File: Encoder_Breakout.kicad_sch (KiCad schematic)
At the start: 4 parts, among them J1 Conn_01x03, J2 Conn_02x07_Odd_Even, J3 Conn_01x02, J4 Conn_01x02

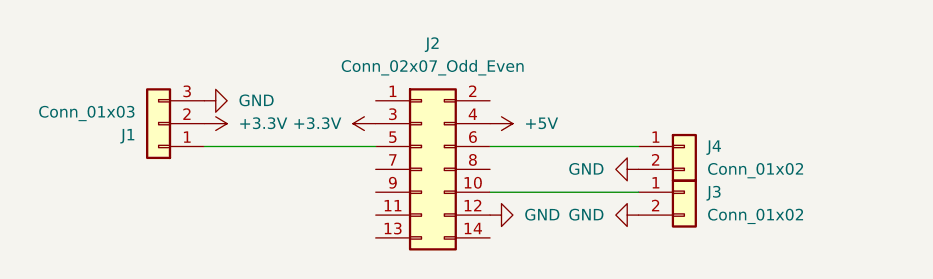
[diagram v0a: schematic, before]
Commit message: PCB changes and add kibot
Signed-off-by: Colin <cfinn68916@gmail.com>
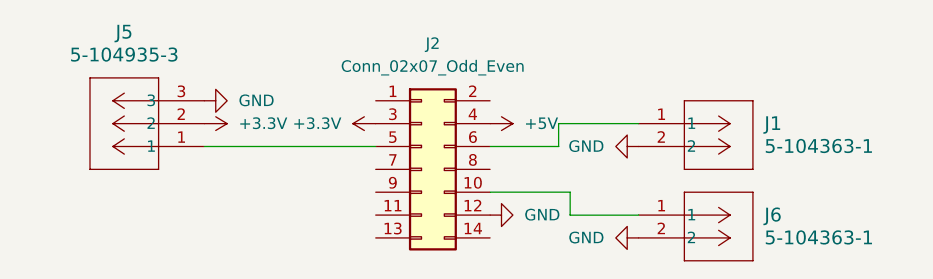
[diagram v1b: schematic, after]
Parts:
- removed J1: Conn_01x03, Connector_PinHeader_2.54mm:PinHeader_1x03_P2.54mm_Horizontal, symbol Connector_Generic:Conn_01x03
- removed J3, J4: Conn_01x02, Connector_PinSocket_2.54mm:PinSocket_1x02_P2.54mm_Vertical, symbol Connector_Generic:Conn_01x02
- added J1, J6: 5-104363-1, CONN_5-104363-1_TYCO, symbol 2023-10-03_23-14-34:5-104363-1
- added J5: 5-104935-3, footprints:CONN_5-104935-3_TYCO, symbol 2023-10-03_22-41-26:5-104935-3
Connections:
- net +3.3V: now also J5.2
- net GND: now also J1.2, J5.3, J6.2
- net at J2.10 (Pin_10): now also J6.1
- net at J2.6 (Pin_6): now also J1.1
- net at J2.5 (Pin_5): now also J5.1
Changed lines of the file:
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@@
 (kicad_sch (version 20230121) (generator eeschema)
   (paper "A4")
-  (wire (pts (xy 146.05 80.01) (xy 162.56 80.01))
+  (wire (pts (xy 154.94 87.63) (xy 162.56 87.63))
+    (stroke (width 0) (type default))
+  )
+  (wire (pts (xy 146.05 80.01) (xy 153.67 80.01))
+    (stroke (width 0) (type default))
+  )
+  (wire (pts (xy 146.05 85.09) (xy 154.94 85.09))
+    (stroke (width 0) (type default))
+  )
+  (wire (pts (xy 154.94 85.09) (xy 154.94 87.63))
+    (stroke (width 0) (type default))
+  )
+  (wire (pts (xy 153.67 80.01) (xy 153.67 77.47))
     (stroke (width 0) (type default))
   )
@@
     (stroke (width 0) (type default))
   )
-  (wire (pts (xy 146.05 85.09) (xy 162.56 85.09))
-    (stroke (width 0) (type default))
-  )
-  (symbol (lib_id "power:GND") (at 162.56 82.55 270) (unit 1)
-    (in_bom yes) (on_board yes) (dnp no) (fields_autoplaced)
-    (property "Reference" "#PWR07" (at 156.21 82.55 0)
-      (effects (font (size 1.27 1.27)) hide)
-    )
-    (property "Value" "GND" (at 158.75 82.55 90)
-      (effects (font (size 1.27 1.27)) (justify right))
-    )
-    (property "Footprint" "" (at 162.56 82.55 0)
-      (effects (font (size 1.27 1.27)) hide)
-    )
-    (property "Datasheet" "" (at 162.56 82.55 0)
+  (wire (pts (xy 153.67 77.47) (xy 162.56 77.47))
+    (stroke (width 0) (type default))
+  )
+  (symbol (lib_id "power:GND") (at 162.56 80.01 270) (unit 1)
+    (in_bom yes) (on_board yes) (dnp no) (fields_autoplaced)
+    (property "Reference" "#PWR07" (at 156.21 80.01 0)
+      (effects (font (size 1.27 1.27)) hide)
+    )
+    (property "Value" "GND" (at 158.75 80.01 90)
+      (effects (font (size 1.27 1.27)) (justify right))
+    )
+    (property "Footprint" "" (at 162.56 80.01 0)
+      (effects (font (size 1.27 1.27)) hide)
+    )
+    (property "Datasheet" "" (at 162.56 80.01 0)
       (effects (font (size 1.27 1.27)) hide)
     )
@@
     )
   )
-  (symbol (lib_id "Connector_Generic:Conn_01x02") (at 167.64 85.09 0) (unit 1)
-    (in_bom yes) (on_board yes) (dnp no) (fields_autoplaced)
-    (property "Reference" "J3" (at 170.18 85.09 0)
-      (effects (font (size 1.27 1.27)) (justify left))
-    )
-    (property "Value" "Conn_01x02" (at 170.18 87.63 0)
-      (effects (font (size 1.27 1.27)) (justify left))
-    )
-    (property "Footprint" "Connector_PinSocket_2.54mm:PinSocket_1x02_P2.54mm_Vertical" (at 167.64 85.09 0)
-      (effects (font (size 1.27 1.27)) hide)
-    )
-    (property "Datasheet" "~" (at 167.64 85.09 0)
-      (effects (font (size 1.27 1.27)) hide)
-    )
-    (pin "1")
-    (pin "2")
-    (instances
-      (project "Encoder_Breakout"
-        (path "/896045ed-d89c-42ad-9d47-a66b46c2187b"
-          (reference "J3") (unit 1)
+  (symbol (lib_id "2023-10-03_23-14-34:5-104363-1") (at 162.56 77.47 0) (unit 1)
+    (in_bom yes) (on_board yes) (dnp no) (fields_autoplaced)
+    (property "Reference" "J1" (at 176.53 77.47 0)
+      (effects (font (size 1.524 1.524)) (justify left))
+    )
+    (property "Value" "5-104363-1" (at 176.53 80.01 0)
+      (effects (font (size 1.524 1.524)) (justify left))
+    )
+    (property "Footprint" "CONN_5-104363-1_TYCO" (at 162.56 77.47 0)
+      (effects (font (size 1.27 1.27) italic) hide)
+    )
+    (property "Datasheet" "5-104363-1" (at 162.56 77.47 0)
+      (effects (font (size 1.27 1.27) italic) hide)
+    )
+    (pin "1")
+    (pin "2")
+    (instances
+      (project "Encoder_Breakout"
+        (path "/896045ed-d89c-42ad-9d47-a66b46c2187b"
+          (reference "J1") (unit 1)
         )
       )
@@
         (path "/896045ed-d89c-42ad-9d47-a66b46c2187b"
           (reference "#PWR05") (unit 1)
-        )
-      )
-    )
-  )
-  (symbol (lib_id "Connector_Generic:Conn_01x02") (at 167.64 80.01 0) (unit 1)
-    (in_bom yes) (on_board yes) (dnp no) (fields_autoplaced)
-    (property "Reference" "J4" (at 170.18 80.01 0)
-      (effects (font (size 1.27 1.27)) (justify left))
-    )
-    (property "Value" "Conn_01x02" (at 170.18 82.55 0)
-      (effects (font (size 1.27 1.27)) (justify left))
-    )
-    (property "Footprint" "Connector_PinSocket_2.54mm:PinSocket_1x02_P2.54mm_Vertical" (at 167.64 80.01 0)
-      (effects (font (size 1.27 1.27)) hide)
-    )
-    (property "Datasheet" "~" (at 167.64 80.01 0)
-      (effects (font (size 1.27 1.27)) hide)
-    )
-    (pin "1")
-    (pin "2")
-    (instances
-      (project "Encoder_Breakout"
-        (path "/896045ed-d89c-42ad-9d47-a66b46c2187b"
-          (reference "J4") (unit 1)
         )
       )
@@
         (path "/896045ed-d89c-42ad-9d47-a66b46c2187b"
           (reference "#PWR04") (unit 1)
-        )
-      )
-    )
-  )
-  (symbol (lib_id "Connector_Generic:Conn_01x03") (at 109.22 77.47 180) (unit 1)
-    (in_bom yes) (on_board yes) (dnp no) (fields_autoplaced)
-    (property "Reference" "J1" (at 106.68 78.74 0)
-      (effects (font (size 1.27 1.27)) (justify left))
-    )
-    (property "Value" "Conn_01x03" (at 106.68 76.2 0)
-      (effects (font (size 1.27 1.27)) (justify left))
-    )
-    (property "Footprint" "Connector_PinHeader_2.54mm:PinHeader_1x03_P2.54mm_Horizontal" (at 109.22 77.47 0)
-      (effects (font (size 1.27 1.27)) hide)
-    )
-    (property "Datasheet" "~" (at 109.22 77.47 0)
-      (effects (font (size 1.27 1.27)) hide)
-    )
-    (pin "1")
-    (pin "2")
-    (pin "3")
-    (instances
-      (project "Encoder_Breakout"
-        (path "/896045ed-d89c-42ad-9d47-a66b46c2187b"
-          (reference "J1") (unit 1)
         )
       )
@@
     )
   )
-  (symbol (lib_id "power:GND") (at 162.56 87.63 270) (unit 1)
-    (in_bom yes) (on_board yes) (dnp no) (fields_autoplaced)
-    (property "Reference" "#PWR06" (at 156.21 87.63 0)
-      (effects (font (size 1.27 1.27)) hide)
-    )
-    (property "Value" "GND" (at 158.75 87.63 90)
-      (effects (font (size 1.27 1.27)) (justify right))
-    )
-    (property "Footprint" "" (at 162.56 87.63 0)
-      (effects (font (size 1.27 1.27)) hide)
-    )
-    (property "Datasheet" "" (at 162.56 87.63 0)
+  (symbol (lib_id "power:GND") (at 162.56 90.17 270) (unit 1)
+    (in_bom yes) (on_board yes) (dnp no) (fields_autoplaced)
+    (property "Reference" "#PWR06" (at 156.21 90.17 0)
+      (effects (font (size 1.27 1.27)) hide)
+    )
+    (property "Value" "GND" (at 158.75 90.17 90)
+      (effects (font (size 1.27 1.27)) (justify right))
+    )
+    (property "Footprint" "" (at 162.56 90.17 0)
+      (effects (font (size 1.27 1.27)) hide)
+    )
+    (property "Datasheet" "" (at 162.56 90.17 0)
       (effects (font (size 1.27 1.27)) hide)
     )
@@
     )
   )
+  (symbol (lib_id "2023-10-03_22-41-26:5-104935-3") (at 114.3 80.01 180) (unit 1)
+    (in_bom yes) (on_board yes) (dnp no) (fields_autoplaced)
+    (property "Reference" "J5" (at 105.41 67.31 0)
+      (effects (font (size 1.524 1.524)))
+    )
+    (property "Value" "5-104935-3" (at 105.41 69.85 0)
+      (effects (font (size 1.524 1.524)))
+    )
+    (property "Footprint" "footprints:CONN_5-104935-3_TYCO" (at 114.3 80.01 0)
+      (effects (font (size 1.27 1.27) italic) hide)
+    )
+    (property "Datasheet" "5-104935-3" (at 114.3 80.01 0)
+      (effects (font (size 1.27 1.27) italic) hide)
+    )
+    (pin "1")
+    (pin "2")
+    (pin "3")
+    (instances
+      (project "Encoder_Breakout"
+        (path "/896045ed-d89c-42ad-9d47-a66b46c2187b"
+          (reference "J5") (unit 1)
+        )
+      )
+    )
+  )
   (symbol (lib_id "power:GND") (at 146.05 87.63 90) (unit 1)
     (in_bom yes) (on_board yes) (dnp no) (fields_autoplaced)
@@
         )
       )
+    )
+  )
+  (symbol (lib_id "2023-10-03_23-14-34:5-104363-1") (at 162.56 87.63 0) (unit 1)
+    (in_bom yes) (on_board yes) (dnp no) (fields_autoplaced)
+    (property "Reference" "J6" (at 176.53 87.63 0)
+      (effects (font (size 1.524 1.524)) (justify left))
+    )
+    (property "Value" "5-104363-1" (at 176.53 90.17 0)
+      (effects (font (size 1.524 1.524)) (justify left))
+    )
+    (property "Footprint" "CONN_5-104363-1_TYCO" (at 162.56 87.63 0)
+      (effects (font (size 1.27 1.27) italic) hide)
+    )
+    (property "Datasheet" "5-104363-1" (at 162.56 87.63 0)
+      (effects (font (size 1.27 1.27) italic) hide)
+    )
+    (pin "1")
+    (pin "2")
+    (instances
+      (project "Encoder_Breakout"
+        (path "/896045ed-d89c-42ad-9d47-a66b46c2187b"
+          (reference "J6") (unit 1)
+        )
+      )
